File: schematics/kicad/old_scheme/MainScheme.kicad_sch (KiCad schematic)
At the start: 12 parts, among them J1 Raspberry Pi 4, U1 L298N

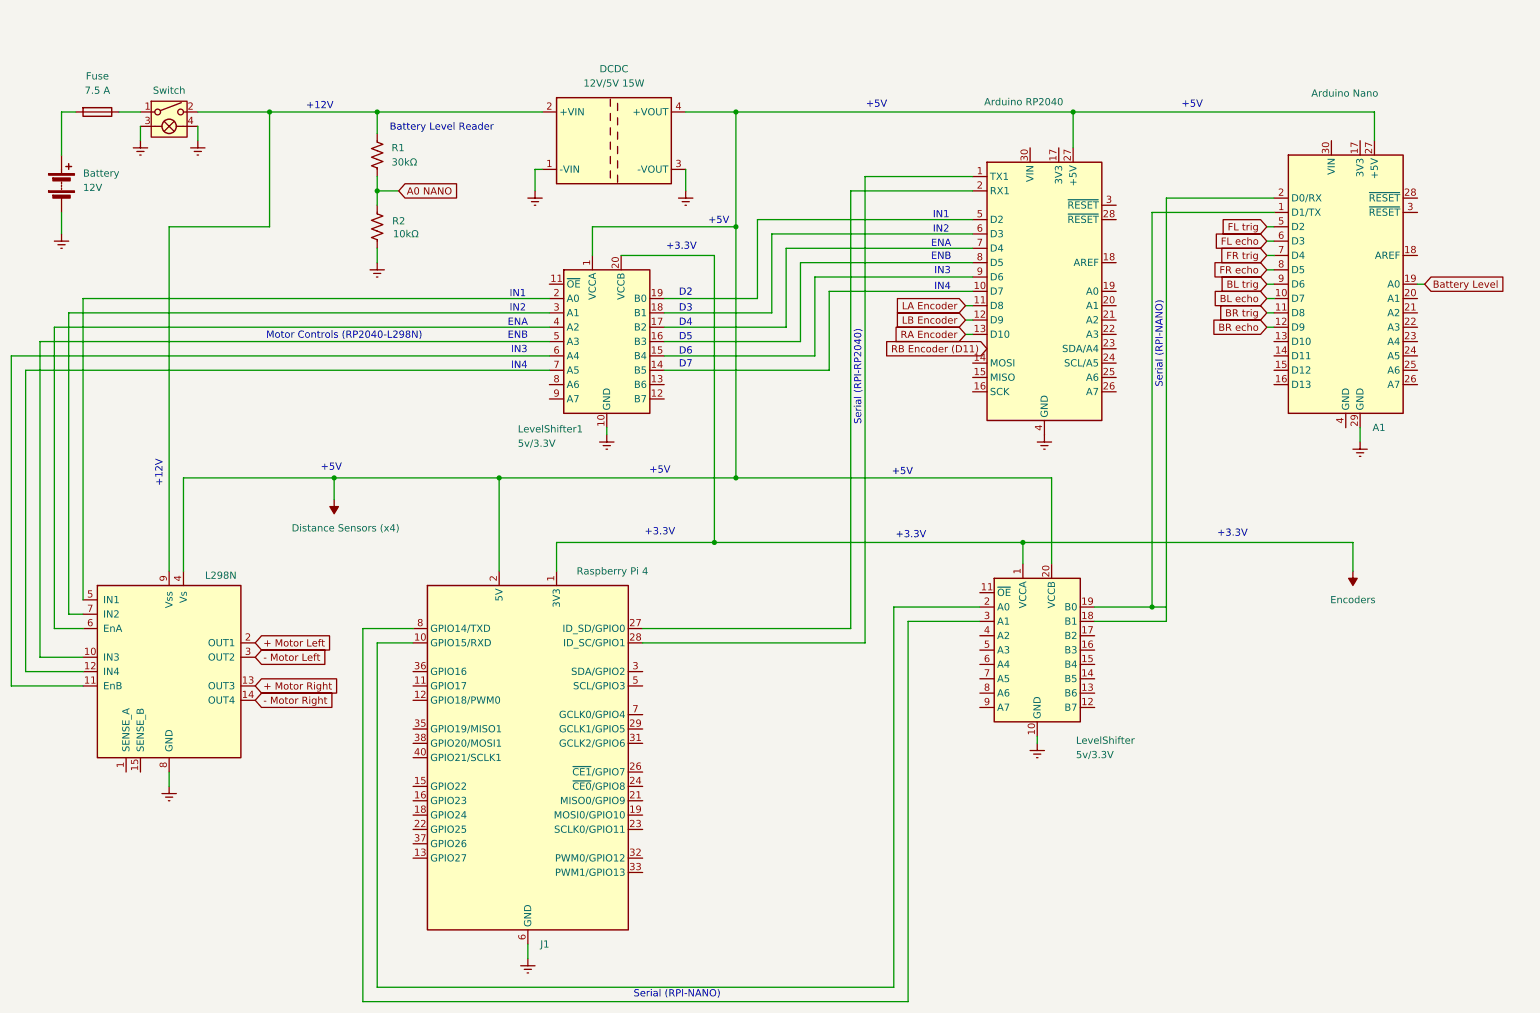
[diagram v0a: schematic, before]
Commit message: update schematics
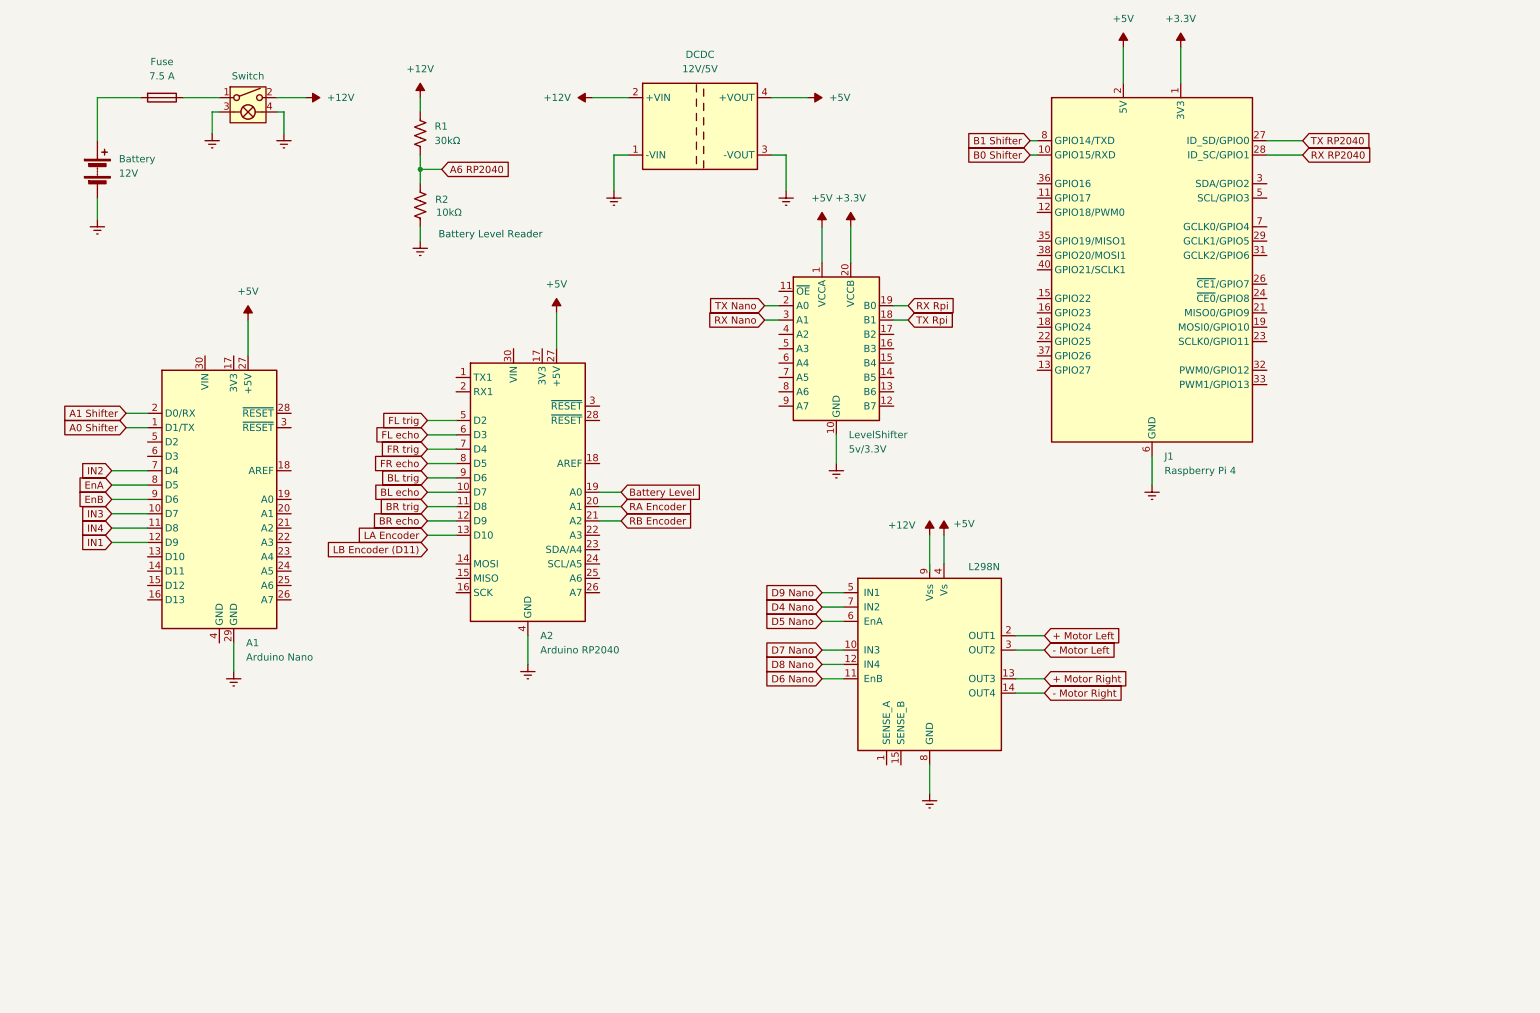
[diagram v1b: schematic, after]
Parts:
- removed LevelShifter1: 5v/3.3V, Package_DFN_QFN:WQFN-20-1EP_2.5x4.5mm_P0.5mm_EP1x2.9mm, symbol Logic_LevelTranslator:FXMA108
- DCDC: value 12V/5V 15W -> 12V/5V
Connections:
- net LB Encoder is gone; now on net BR echo: A2.12 (D9)
- net BL echo: now also A2.10 (D7); no longer A1.10 (D7)
- net BL trig: now also A2.9 (D6); no longer A1.9 (D6)
- net BR echo: no longer A1.12 (D9)
- net BR trig: now also A2.11 (D8); no longer A1.11 (D8)
- net Battery Level: now also A2.19 (A0); no longer A1.19 (A0)
- net FL echo: now also A2.6 (D3); no longer A1.6 (D3)
- net FL trig: now also A2.5 (D2); no longer A1.5 (D2)
- net FR echo: now also A2.8 (D5); no longer A1.8 (D5)
- net FR trig: now also A2.7 (D4); no longer A1.7 (D4)
- net LA Encoder: now also A2.13 (D10); no longer A2.11 (D8)
- net RA Encoder: now also A2.20 (A1); no longer A2.13 (D10)
- net D7 Nano: now reaches U1.10 (IN3)
- net D6 Nano: now reaches U1.11 (EnB)
- net D8 Nano: now reaches U1.12 (IN4)
- net D9 Nano: now reaches U1.5 (IN1)
- net D5 Nano: now reaches U1.6 (EnA)
- net D4 Nano: now reaches U1.7 (IN2)
- net +12V: now reaches DCDC.2 (+VIN), R1.2, dsd.2
- net +12V: no longer U1.9 (Vss)
- net A1 Shifter: now reaches A1.2 (D0/RX)
- net A1 Shifter: no longer LevelShifter.18 (B1)
- net A0 Shifter: now reaches A1.1 (D1/TX)
- net A0 Shifter: no longer LevelShifter.19 (B0)
- net B0 Shifter: now reaches J1.10 (GPIO15/RXD)
- net B0 Shifter: no longer LevelShifter.2 (A0)
- net B1 Shifter: now reaches J1.8 (GPIO14/TXD)
- net B1 Shifter: no longer LevelShifter.3 (A1)
- net at A2.1 (TX1): no longer J1.28 (ID_SC/GPIO1)
- net at A2.2 (RX1): no longer J1.27 (ID_SD/GPIO0)
- net RB Encoder: now reaches A2.21 (A2)
- net A0 NANO renamed A6 RP2040
- net Distance Sensors (x4) renamed +5V
- net +5V: now also LevelShifter.1 (VCCA); no longer LevelShifter.20 (VCCB)
- net Encoders renamed +3.3V
- net +3.3V: now also LevelShifter.20 (VCCB); no longer LevelShifter.1 (VCCA)
- new net EnA: A1.8 (D5)
- new net EnB: A1.9 (D6)
- new net IN1: A1.12 (D9)
- new net IN2: A1.7 (D4)
- new net IN3: A1.10 (D7)
- new net IN4: A1.11 (D8)
- new net RX Nano: LevelShifter.3 (A1)
- new net RX RP2040: J1.28 (ID_SC/GPIO1)
- new net RX Rpi: LevelShifter.19 (B0)
- new net TX Nano: LevelShifter.2 (A0)
- new net TX RP2040: J1.27 (ID_SD/GPIO0)
- new net TX Rpi: LevelShifter.18 (B1)
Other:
- note removed: "+12V"
- note removed: "+3.3V"
- note removed: "+5V"
- note removed: "D2"
- note removed: "D3"
- note removed: "D4"
- note removed: "D5"
- note removed: "D6"
- note removed: "D7"
- note removed: "ENA"
- note removed: "ENB"
- note removed: "IN1"
- note removed: "IN2"
- note removed: "IN3"
- note removed: "IN4"
- note removed: "Motor Controls (RP2040-L298N)"
- note removed: "Serial (RPI-NANO)"
- note removed: "Serial (RPI-RP2040)"
- moved on the sheet: A1, Battery, DCDC, Fuse, J1, LevelShifter, R1, R2
